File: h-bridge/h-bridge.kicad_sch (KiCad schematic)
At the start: 32 parts, among them Q1 IRF4905, Q2 IRLZ44N, Q3 IRF4905, Q4 IRLZ44N, Q5 2N2222, Q6 2N2222, Q7 IRF4905, Q8 IRF4905

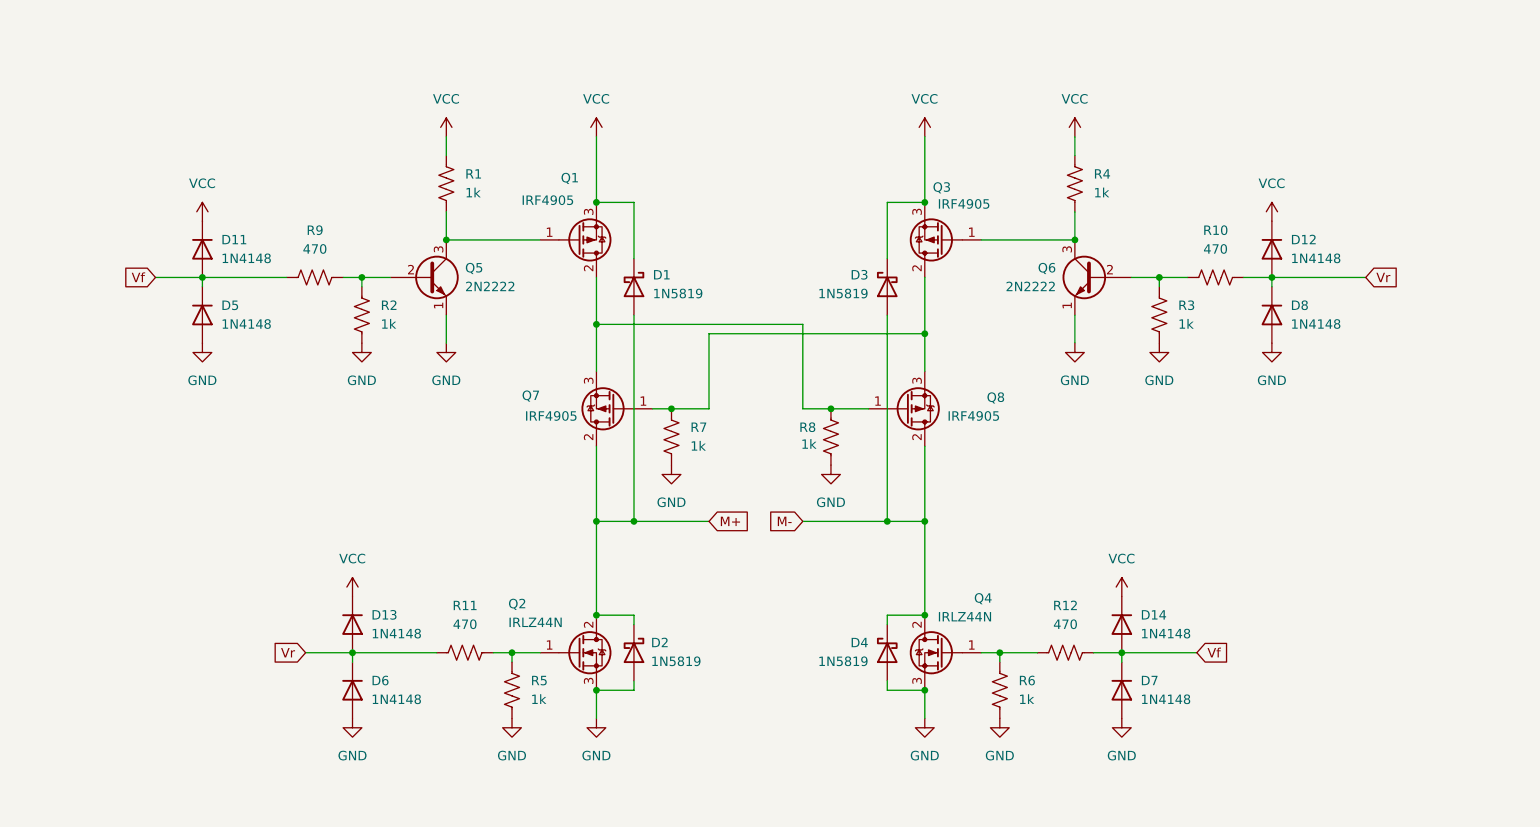
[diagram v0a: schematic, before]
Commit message: Updated BOM
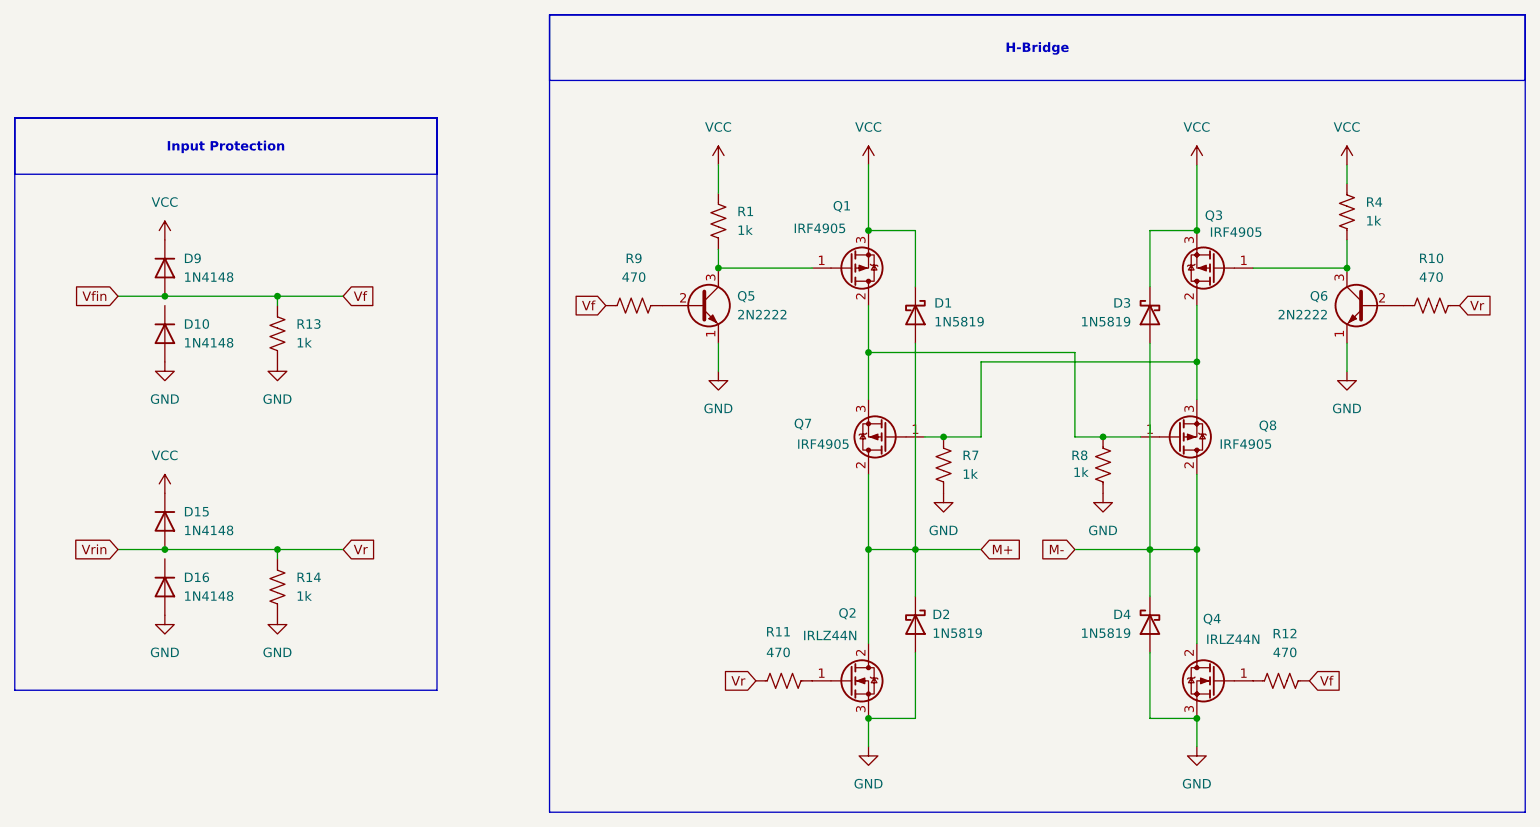
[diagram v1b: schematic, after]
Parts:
- removed D11, D12, D13, D14, D5, D6, D7, D8: 1N4148, Diode_THT:D_DO-35_SOD27_P7.62mm_Horizontal, symbol Diode:1N4148
- removed R2, R3, R5, R6: 1k, symbol Device:R_US
- added D10, D15, D16, D9: 1N4148, Diode_THT:D_DO-35_SOD27_P7.62mm_Horizontal, symbol Diode:1N4148
- added R13, R14: 1k, symbol Device:R_US
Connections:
- net GND: now also D10.2 (A), D16.2 (A), R13.2, R14.2
- net VCC: now also D15.1 (K), D9.1 (K)
- net Vf: now also D9.2 (A), R13.1
- net Vr: now also D15.2 (A), R14.1
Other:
- moved on the sheet: D1, D2, D3, D4, Q1, Q2, Q3, Q4, Q5, Q6, Q7, Q8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
